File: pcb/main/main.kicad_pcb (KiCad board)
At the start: 2 copper layers, 70 x 65 mm, 102 parts, among them J1 UART, J101 USB_C_Receptacle_USB2.0_16P, J2 JTAG, J3 JTAG SRC, J4 26 pin IDC, J5 Conn_01x06, J6 I2C, Q101 Q_Dual_PMOS_S1G1S2G2D2D2D1D1, Q122 DMP3099L, Q131 FDC6312P, SW1 Boot, SW2 Reset, U1 74LVC1G17, U101 USBLC6-2SC6, U102 TS3USB221A, U103 CYPD3176, U121 TPS63070, U131 TPS629203, U2 74LVC1G17, U3 ESP32-S3-WROOM-1

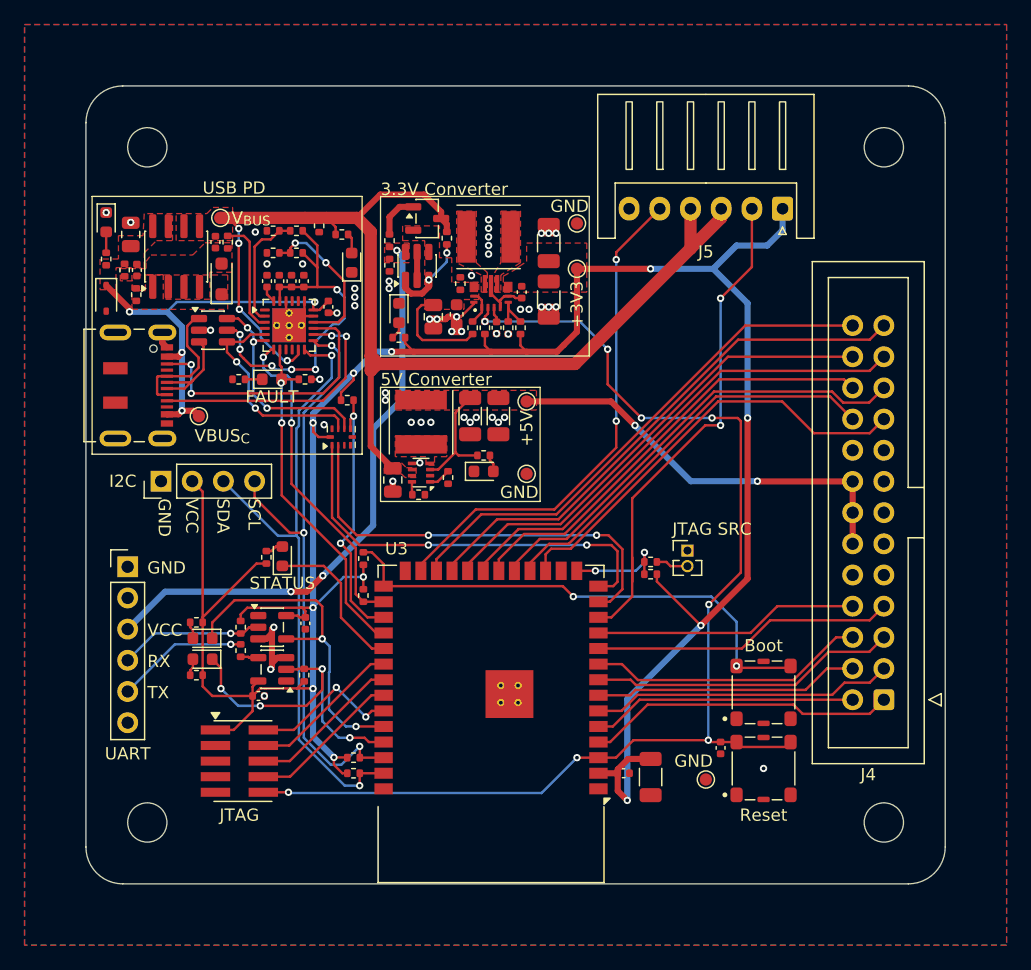
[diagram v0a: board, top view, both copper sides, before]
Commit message: Parts updates, a few board tweaks
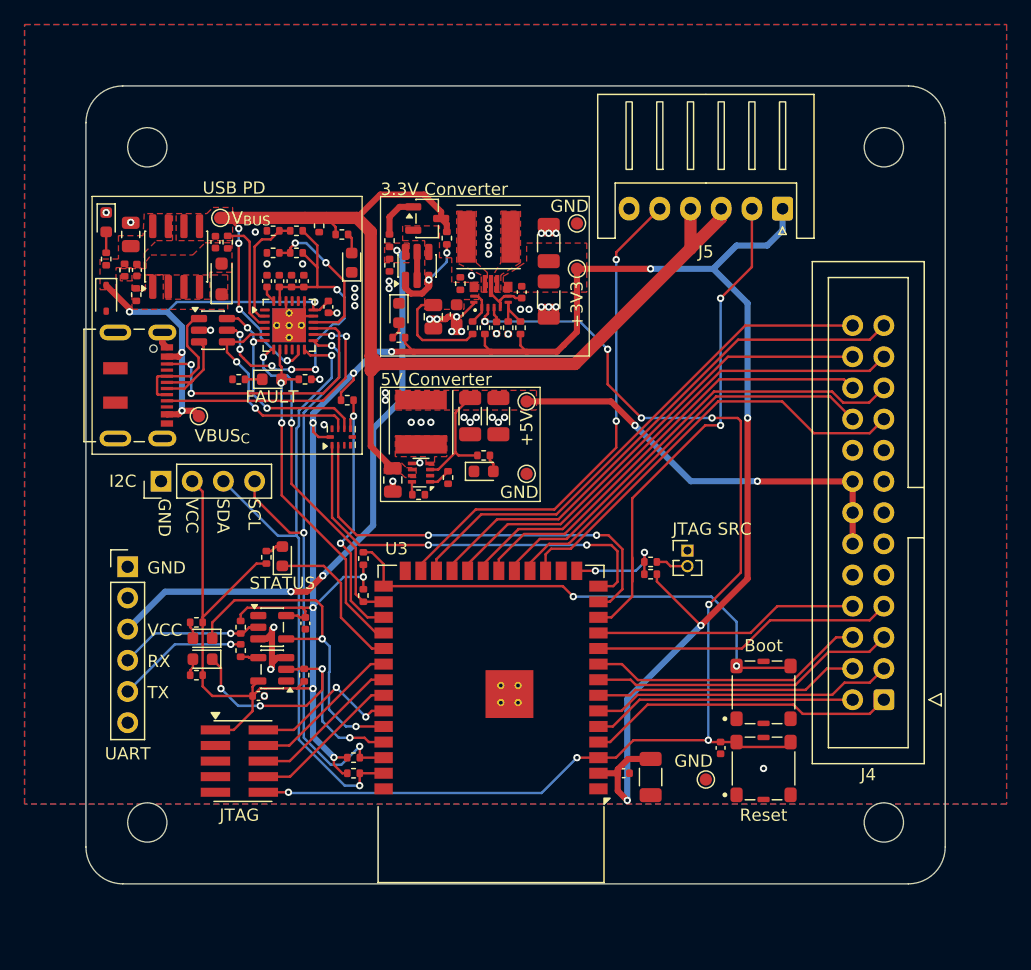
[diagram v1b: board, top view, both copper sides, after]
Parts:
- R104: value 49.9K -> 100k
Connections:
- net /3v3/FB_{3.3V} renamed /3v3/FB_{3V3}
- net /3v3/L1_{3.3V} renamed /3v3/SW_{3V3A}
- net /3v3/L2_{3.3V} renamed /3v3/SW_{3V3B}
- net /3v3/VAUX_{3.3V} renamed /3v3/V_{AUX}
- net /3v3/VIN_{3.3V} renamed /3v3/V_{IN3.3V}
- net /5v/MODE_{5V} renamed /5v/FB_{MODE}
- net /5v/VSET_{5V} renamed /5v/FB_{5V}
- net /usb/GATE renamed /usb/G_{USB}
- net /usb/SOURCE renamed /usb/S_{USB}
- net /usb/VBUS_{C} renamed /usb/V_{BUSC}
- net Net-(U103-ISNK_FINE) renamed /usb/FB_{ISINKF}
- net Net-(U103-VBUS_MAX) renamed /usb/FB_{VBUSMAX}
- net Net-(U103-VCCD) renamed /usb/V_{CCD}
- net VCC_{UART} renamed V_{UART}
- net VDDD renamed V_{DDD}
